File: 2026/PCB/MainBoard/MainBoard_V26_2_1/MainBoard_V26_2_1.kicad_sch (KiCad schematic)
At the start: 94 parts, among them J1 Raspberry_Pi_2_3, J13 //Drib, J15 TFT3, J16 CAN_CON, J2 fan, J3 MOLEX, J5 Conn_01x05_Socket, J6 Debug, Q1 Q_NMOS_GSD, Q2 Q_NMOS_GSD, Q3 Q_NMOS_GSD, SW1 SW_MEC_5E, SW2 Ras_1, SW3 Ras_2, U1 STM32F446RETx, U2 LMR51460FSQDRRRQ1, U3 MOUDLE-SEEEDUINO-XIAO, U5 MCP1703AT-3302E/CB, U6 LSM6DSO32XTR, U7 LTC4451AV-TRPBF, U8 MAX3051, U9 LTC4451AV-TRPBF, Y1 CSTNE16M0V530000R0

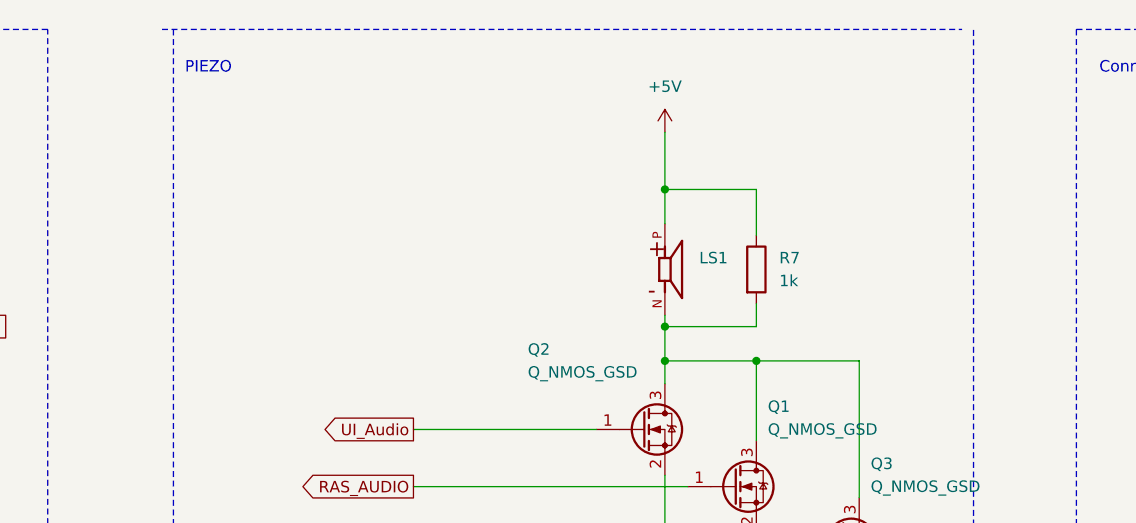
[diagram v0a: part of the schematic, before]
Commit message: 途中保存2
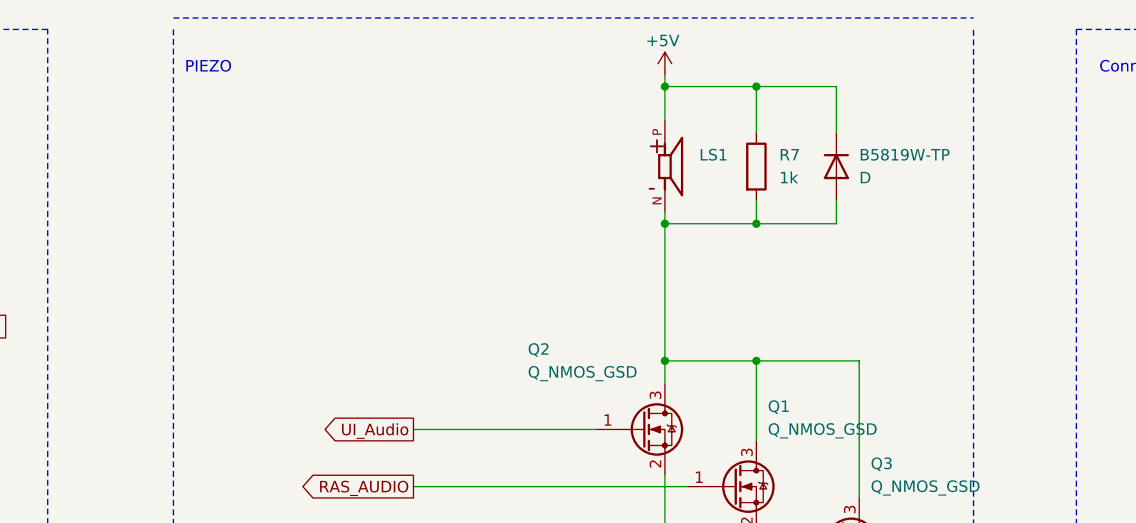
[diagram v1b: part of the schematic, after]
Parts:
- added B5819W-TP: D, symbol Device:D
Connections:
- net +5V: now also B5819W-TP.1 (K)
- net at LS1.N, Q1.3 (D), Q2.3 (D)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: now also B5819W-TP.2 (A)
